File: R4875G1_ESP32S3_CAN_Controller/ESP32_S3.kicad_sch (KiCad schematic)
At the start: 17 parts, among them J1 USB_C_Receptacle_USB2.0_16P, J4 SKU:27579, SW1 SW_Push, SW2 SW_Push, U1 ESP32-S3-WROOM-1

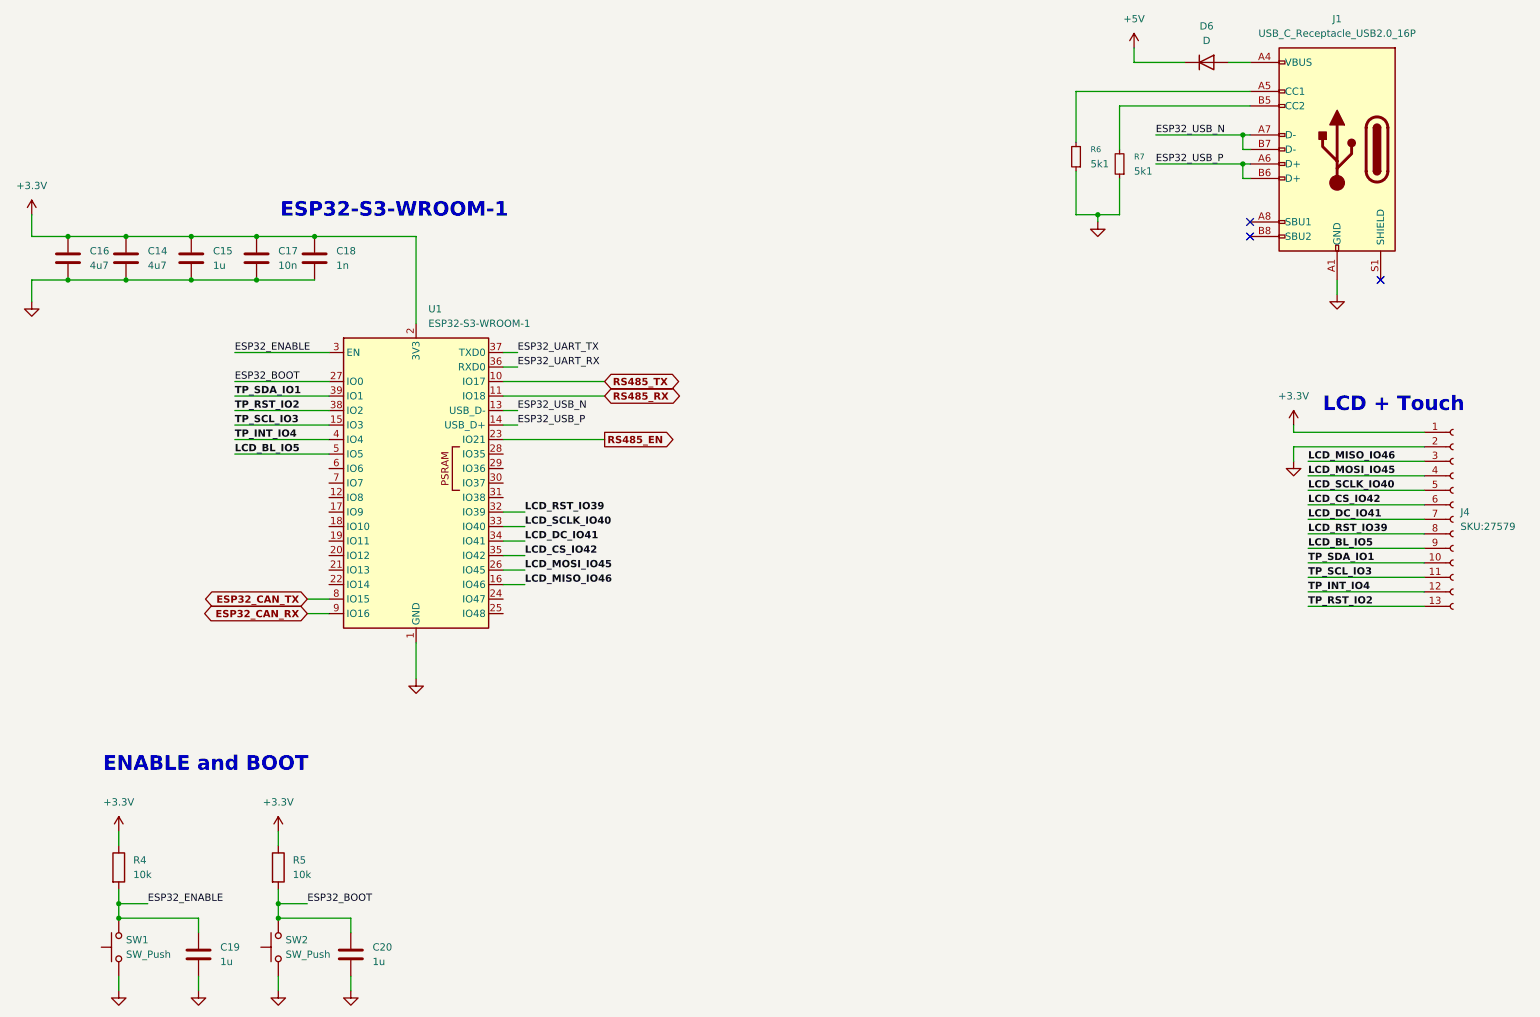
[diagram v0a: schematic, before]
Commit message: Added Kicad files
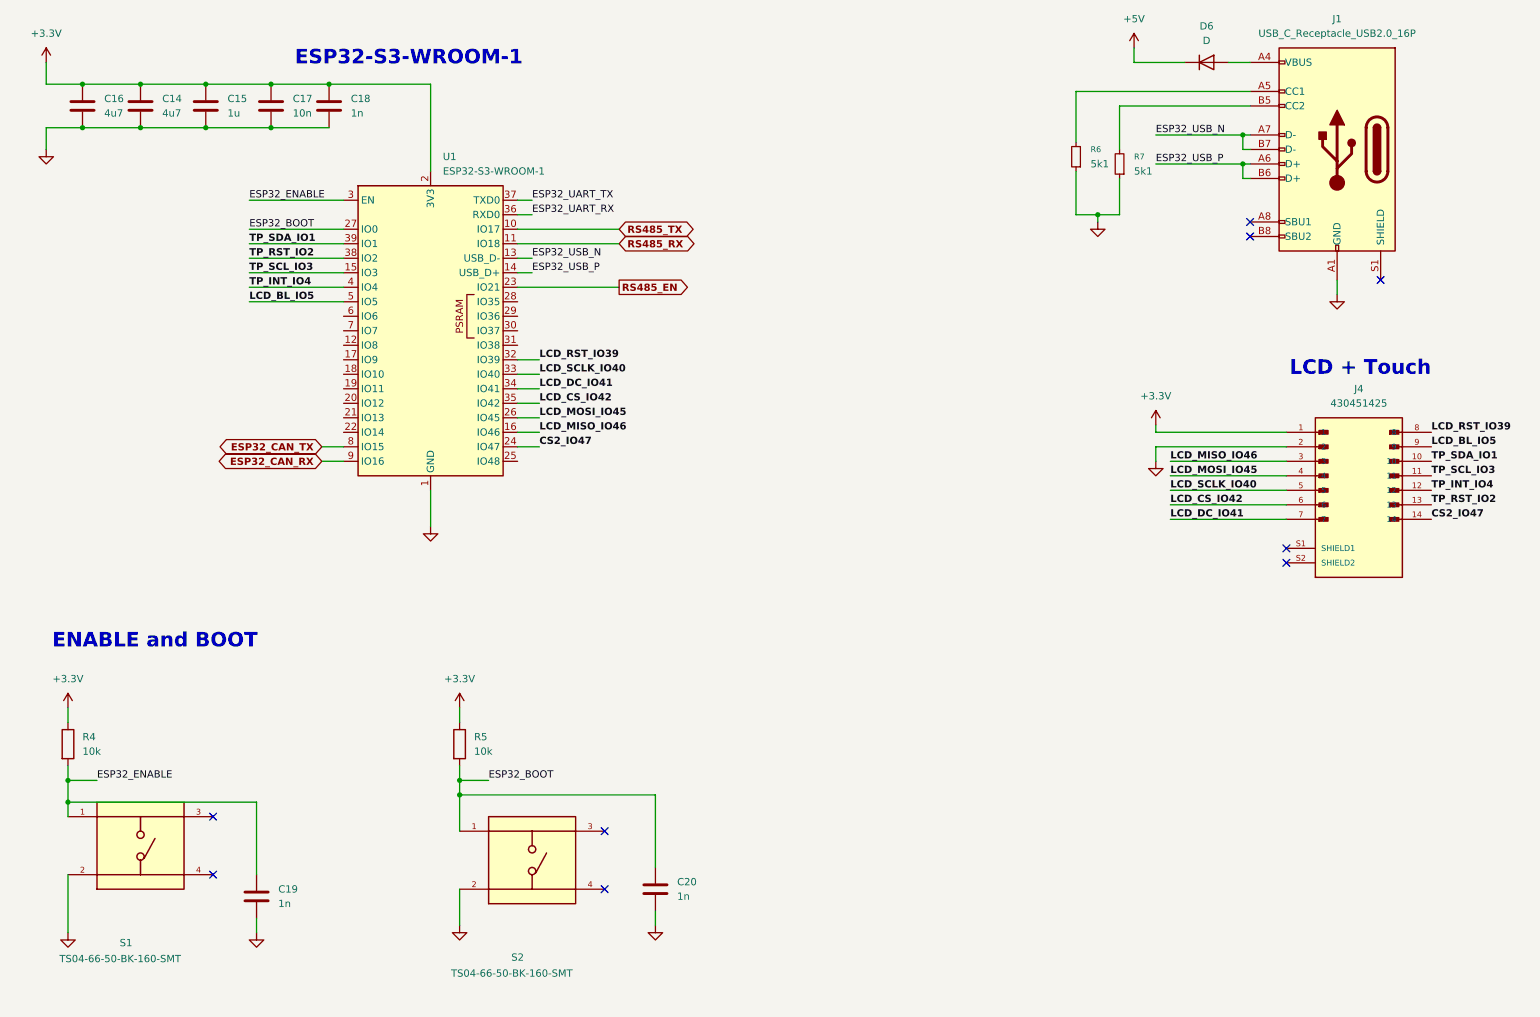
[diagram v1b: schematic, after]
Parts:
- removed J4: SKU:27579, symbol Connector:Conn_01x13_Socket
- removed SW1, SW2: SW_Push, symbol Switch:SW_Push
- added J4: 430451425, 1.0 Added library:MOLEX_430451425, symbol 1.0 Added library:430451425
- added S1, S2: TS04-66-50-BK-160-SMT, 1.0 Added library:SW_TS04-66-50-BK-160-SMT, symbol 1.0 Downloaded models:TS04-66-50-BK-160-SMT
- C14: footprint (none) -> Capacitor_SMD:C_0603_1608Metric_Pad1.08x0.95mm_HandSolder
- C15: footprint (none) -> Capacitor_SMD:C_1210_3225Metric_Pad1.33x2.70mm_HandSolder
- C16: footprint (none) -> Capacitor_SMD:C_0603_1608Metric_Pad1.08x0.95mm_HandSolder; ArosID (none) -> C0683
- C17: footprint (none) -> Capacitor_SMD:C_0805_2012Metric_Pad1.18x1.45mm_HandSolder; ArosID (none) -> C0217
- C18: footprint (none) -> Capacitor_SMD:C_0805_2012Metric_Pad1.18x1.45mm_HandSolder; ArosID (none) -> C0434
- C19: value 1u -> 1n; footprint (none) -> Capacitor_SMD:C_0805_2012Metric_Pad1.18x1.45mm_HandSolder; ArosID (none) -> C0733
- C20: value 1u -> 1n; footprint (none) -> Capacitor_SMD:C_0805_2012Metric_Pad1.18x1.45mm_HandSolder
- D6: footprint (none) -> 1.0 Added library:DIOM5126X265N; ArosID (none) -> D0114
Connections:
- net +3.3V: now also J4.1
- net ESP32_BOOT: now also S2.1
- net ESP32_ENABLE: now also S1.1
- net GND: now also J4.2, S1.2, S2.2
- net LCD_BL_IO5: now also J4.9
- net LCD_CS_IO42: now also J4.6
- net LCD_DC_IO41: now also J4.7
- net LCD_MISO_IO46: now also J4.3
- net LCD_MOSI_IO45: now also J4.4
- net LCD_RST_IO39: now also J4.8
- net LCD_SCLK_IO40: now also J4.5
- net TP_INT_IO4: now also J4.12
- net TP_RST_IO2: now also J4.13
- net TP_SCL_IO3: now also J4.11
- net TP_SDA_IO1: now also J4.10
- net CS2_IO47: now reaches U1.24 (IO47)
- net CS2_IO47: now also J4.14
- no-connect marks 3 -> 9
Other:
- moved on the sheet: C14, C15, C16, C17, C18, C19, C20, R4, R5, U1
